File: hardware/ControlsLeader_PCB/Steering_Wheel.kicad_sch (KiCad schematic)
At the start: 5 parts, among them J10 Indicator_Switch, J8 Conn_01x02_Pin, Q6 NMOS

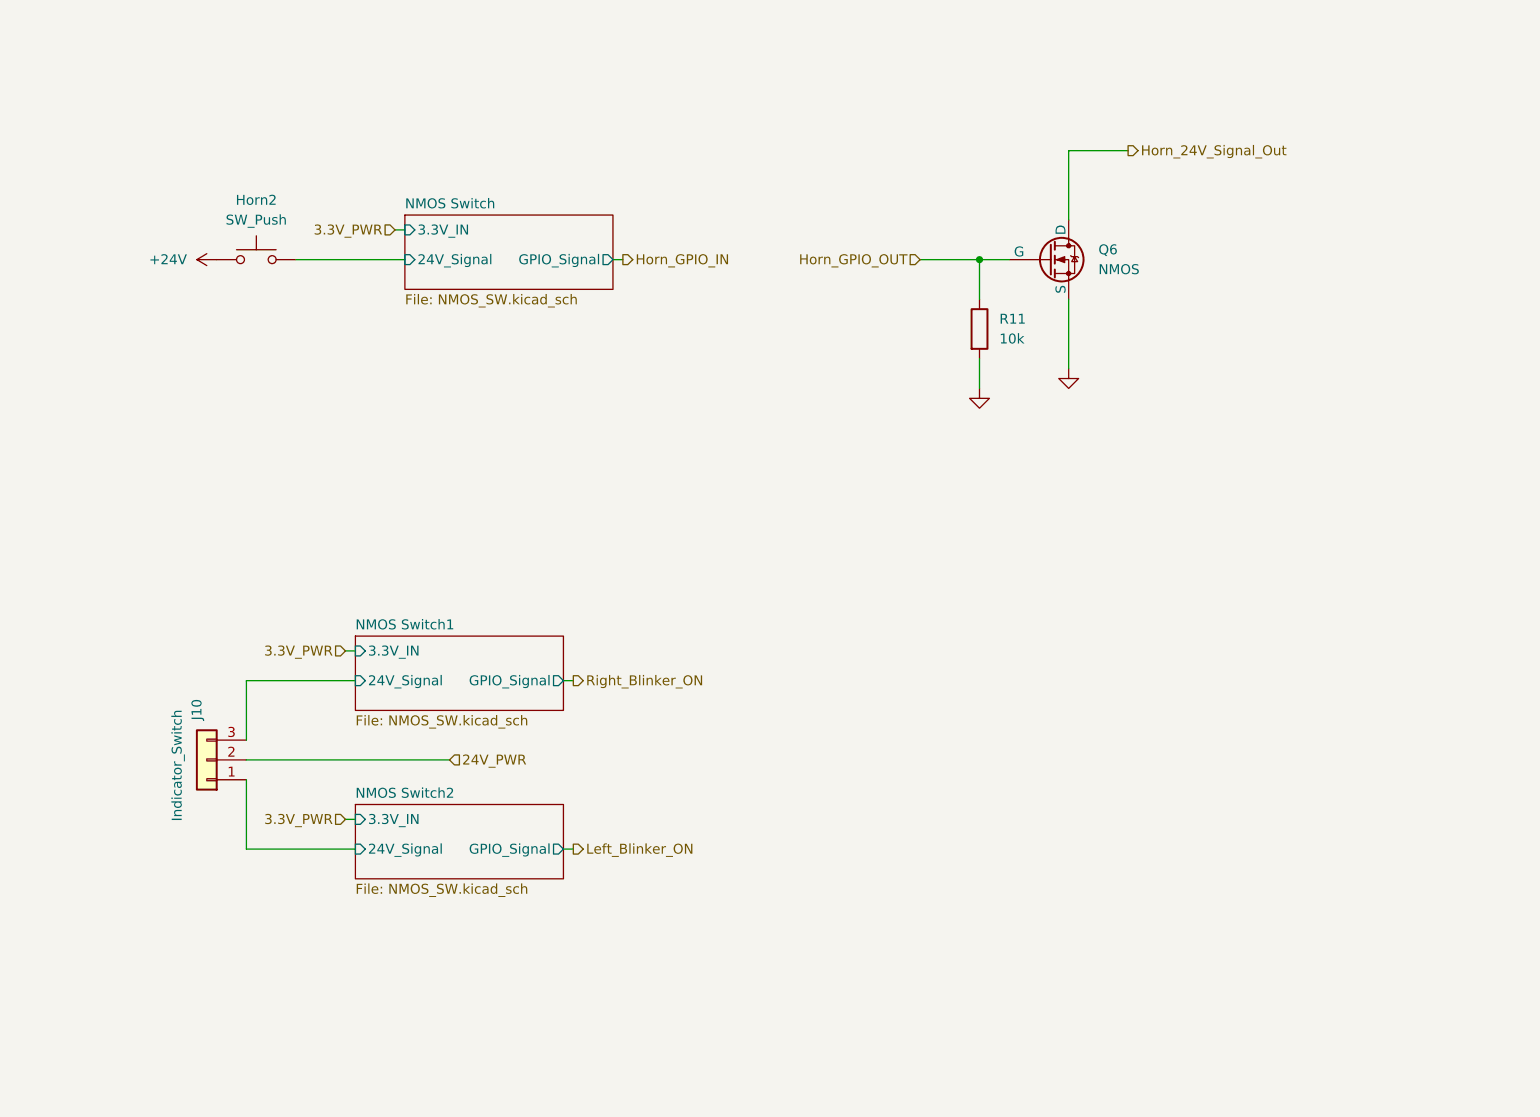
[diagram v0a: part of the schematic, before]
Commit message: DONE!!! - just need to add footprints + part #s)
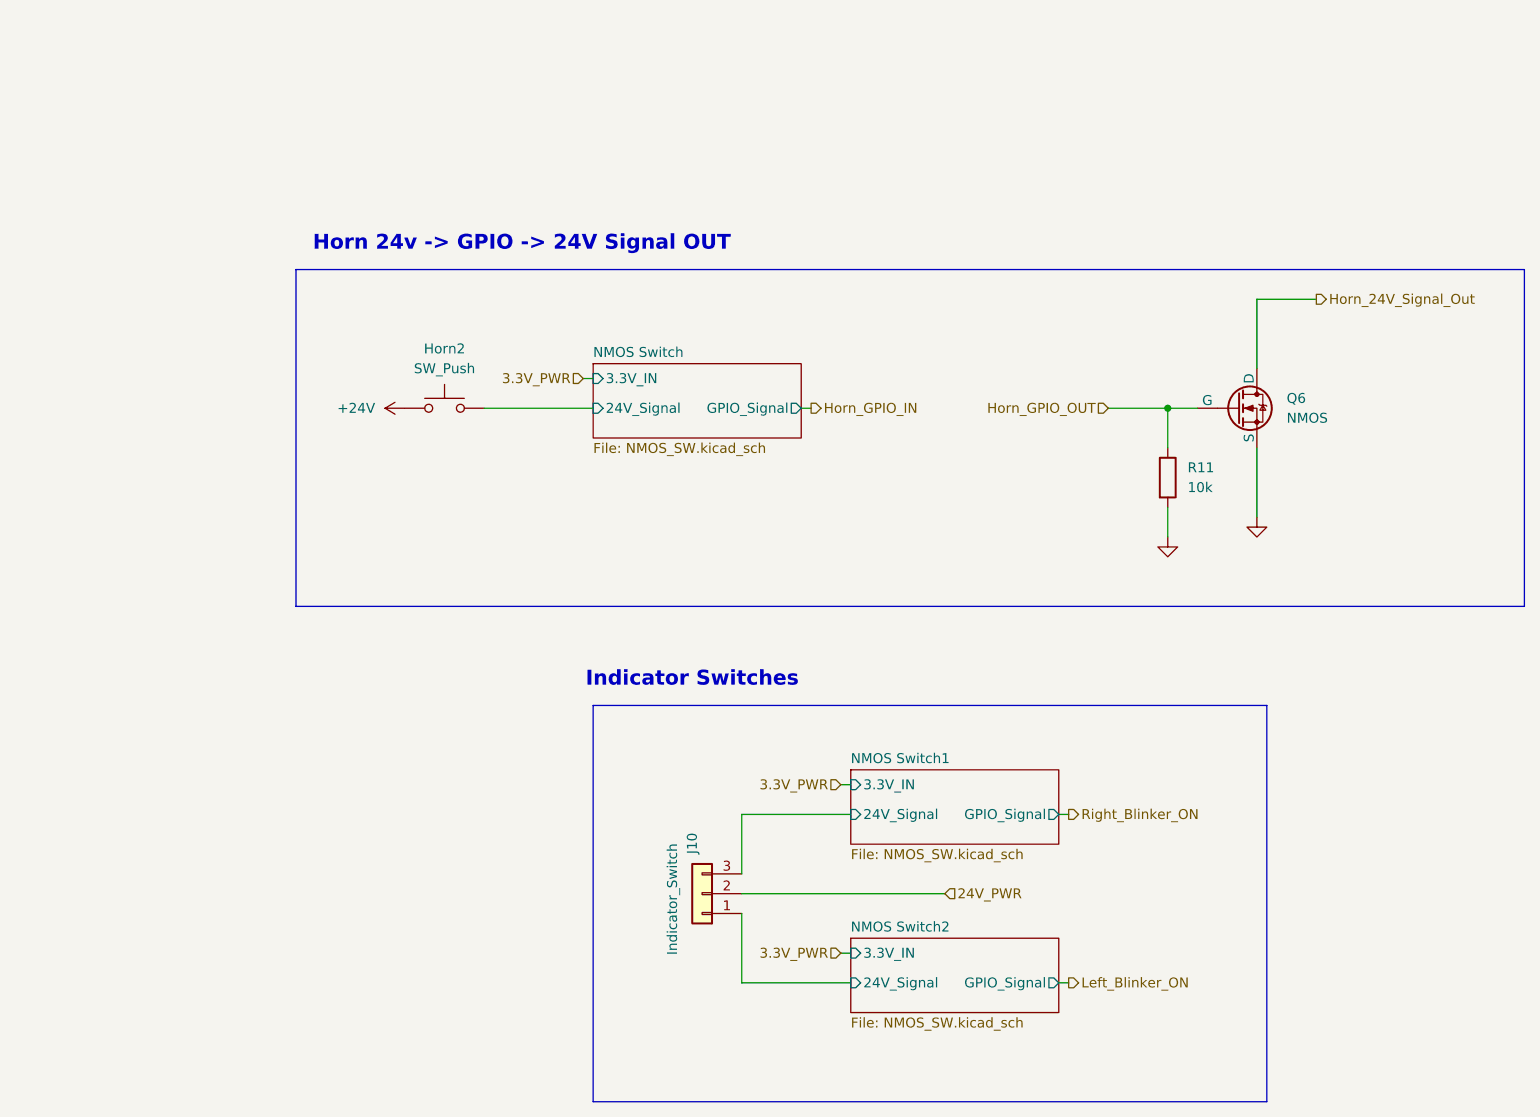
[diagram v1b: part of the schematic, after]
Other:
- note added: "Horn 24v -> GPIO -> 24V Signal OUT"
- note added: "Indicator Switches"
- moved on the sheet: Horn2, J10, Q6, R11
